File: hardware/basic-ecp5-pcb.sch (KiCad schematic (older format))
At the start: 62 parts, among them J1 Conn_01x02, J2 Conn_02x20_Odd_Even, J3 Conn_02x06_Odd_Even, J4 Conn_02x06_Odd_Even, J5 Conn_02x06_Odd_Even, J6 Conn_02x06_Odd_Even, J7 Conn_02x06_Odd_Even, J8 Conn_02x06_Odd_Even, J9 Conn_02x20_Odd_Even, Q1 Q_NMOS_GSD, SW1 SW_Push, SW2 SW_Push, U2 IS25LP016D-JBLE, U3 TLV73311PDBV, U4 TLV73333PDBV, U5 TLV73325PDBV, X1 SiT2001B

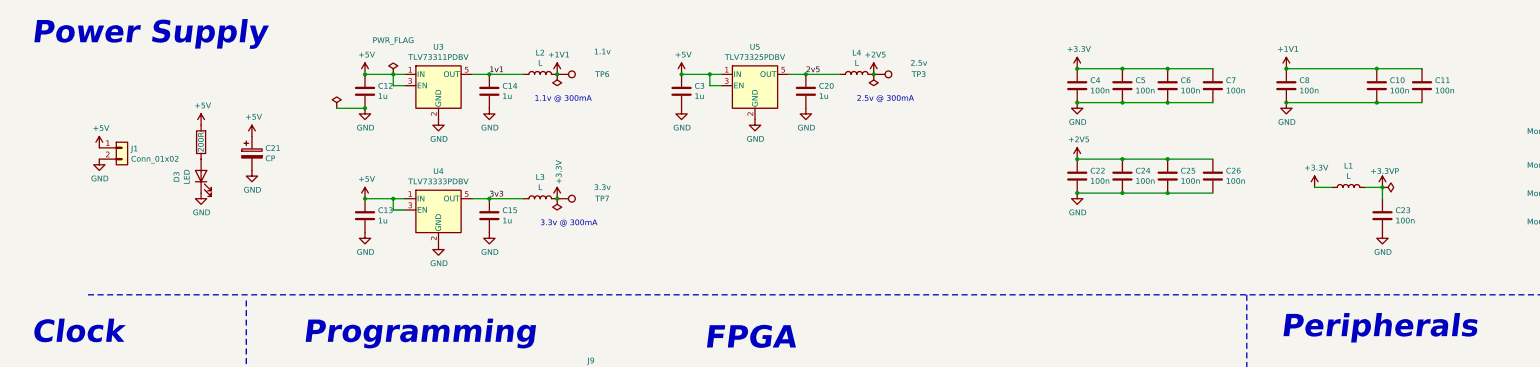
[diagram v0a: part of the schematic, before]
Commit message: changes for design review (see readme)
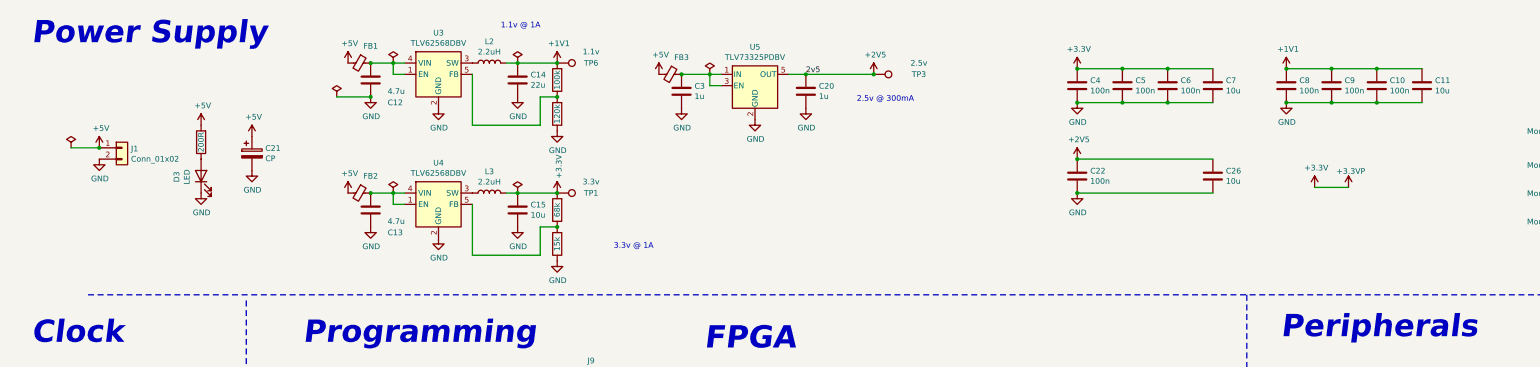
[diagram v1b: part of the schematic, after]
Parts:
- removed C23, C24, C25: 100n, Capacitor_SMD:C_0805_2012Metric, symbol Device:C
- removed L1, L4: L, Inductor_SMD:L_0805_2012Metric, symbol Device:L
- removed TP7: 3.3v, TestPoint:TestPoint_THTPad_D1.0mm_Drill0.5mm, symbol Connector:TestPoint
- removed U3: TLV73311PDBV, Package_TO_SOT_SMD:SOT-23-5, symbol Regulator_Linear:TLV73312PDBV
- removed U4: TLV73333PDBV, Package_TO_SOT_SMD:SOT-23-5, symbol Regulator_Linear:TLV73333PDBV
- added C9: 100n, Capacitor_SMD:C_0805_2012Metric, symbol Device:C
- added FB1, FB2, FB3: Ferrite_Bead_Small, Inductor_SMD:L_0805_2012Metric, symbol Device:Ferrite_Bead_Small
- added R4: 100k, Resistor_SMD:R_0805_2012Metric, symbol Device:R
- added R5: 120k, Resistor_SMD:R_0805_2012Metric, symbol Device:R
- added R7: 68k, Resistor_SMD:R_0805_2012Metric, symbol Device:R
- added R8: 15k, Resistor_SMD:R_0805_2012Metric, symbol Device:R
- added TP1: 3.3v, TestPoint:TestPoint_THTPad_D1.0mm_Drill0.5mm, symbol Connector:TestPoint
- added U3, U4: TLV62568DBV, Package_TO_SOT_SMD:SOT-23-5, symbol Regulator_Switching:TLV62568DBV
- C11, C26, C7: value 100n -> 10u
- C12, C13: value 1u -> 4.7u
- C14: value 1u -> 22u
- C15: value 1u -> 10u
- L2, L3: value L -> 2.2uH; footprint Inductor_SMD:L_0805_2012Metric -> Inductor_SMD:L_Taiyo-Yuden_NR-40xx
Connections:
- net +3V3 is gone; now on net +3.3VP: C1.1, C2.1, C4.1, C5.1, C6.1, C7.1, D1.2 (A), L3.2, R1.1, R10.2, R11.2, R12.2, R13.2, R2.1, U2.8 (VCC), X1.3 (OE), X1.4 (Vcc)
- net 2v5 is gone; now on net +2V5: C20.1, U5.5 (OUT)
- net +1V1: now also C14.1, C9.1, R4.2
- net +3.3VP: now also C15.1, R7.2, TP1.1
- net +5V: now also FB1.2, FB2.2, FB3.2; no longer C12.1, C13.1, C3.1, U5.1 (IN), U5.3 (EN)
- net GND: now also C9.2, R5.1, R8.1, U3.2 (GND), U4.2 (GND)
- net 1v1: no longer names the net of L2.1
- net 1v1: now also U3.3 (SW); no longer C14.1
- net 3v3: no longer names the net of L3.1
- net 3v3: now also U4.3 (SW); no longer C15.1
- new net: C12.1, FB1.1, U3.1 (EN), U3.4 (VIN)
- new net: C3.1, FB3.1, U5.1 (IN), U5.3 (EN)
- new net: R4.1, R5.2, U3.5 (FB)
- new net: C13.1, FB2.1, U4.1 (EN), U4.4 (VIN)
- new net: R7.1, R8.2, U4.5 (FB)
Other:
- note added: "1.1v @ 1A\n"
- note added: "3.3v @ 1A\n"
- note removed: "1.1v @ 300mA"
- note removed: "3.3v @ 300mA"
- moved on the sheet: C12, C14, TP6
